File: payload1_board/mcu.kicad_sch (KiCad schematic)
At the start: 34 parts, among them U1 STM32WLE5CCU6, Y1 32.768KHz, Y2 32MHz

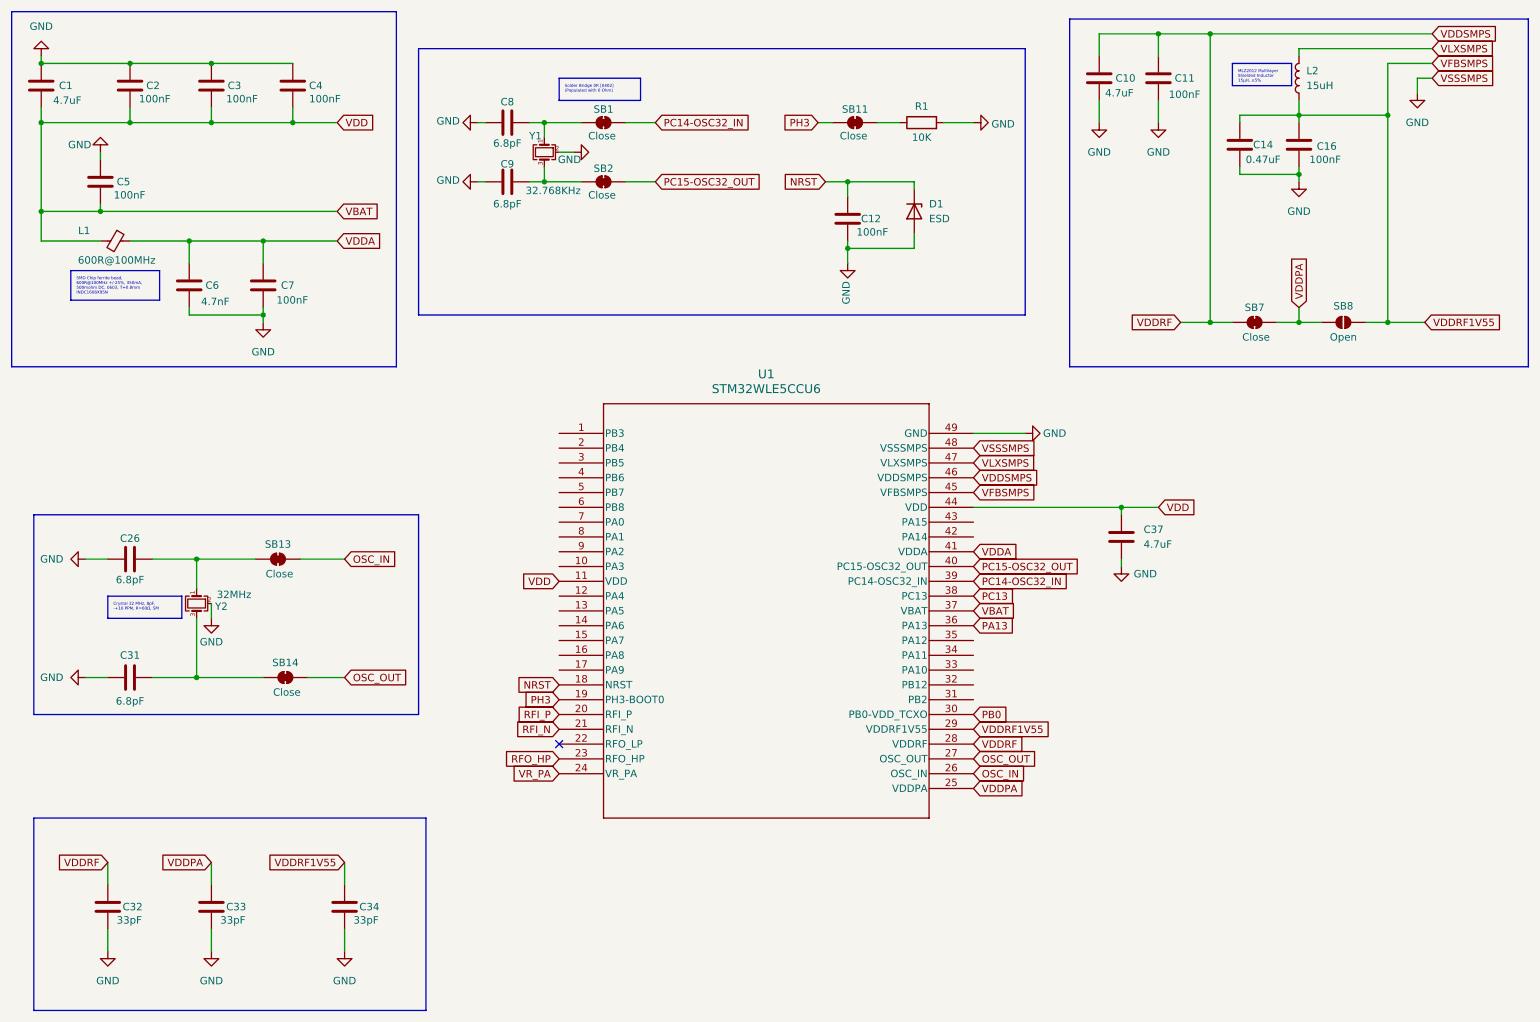
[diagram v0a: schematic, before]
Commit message: sensors done
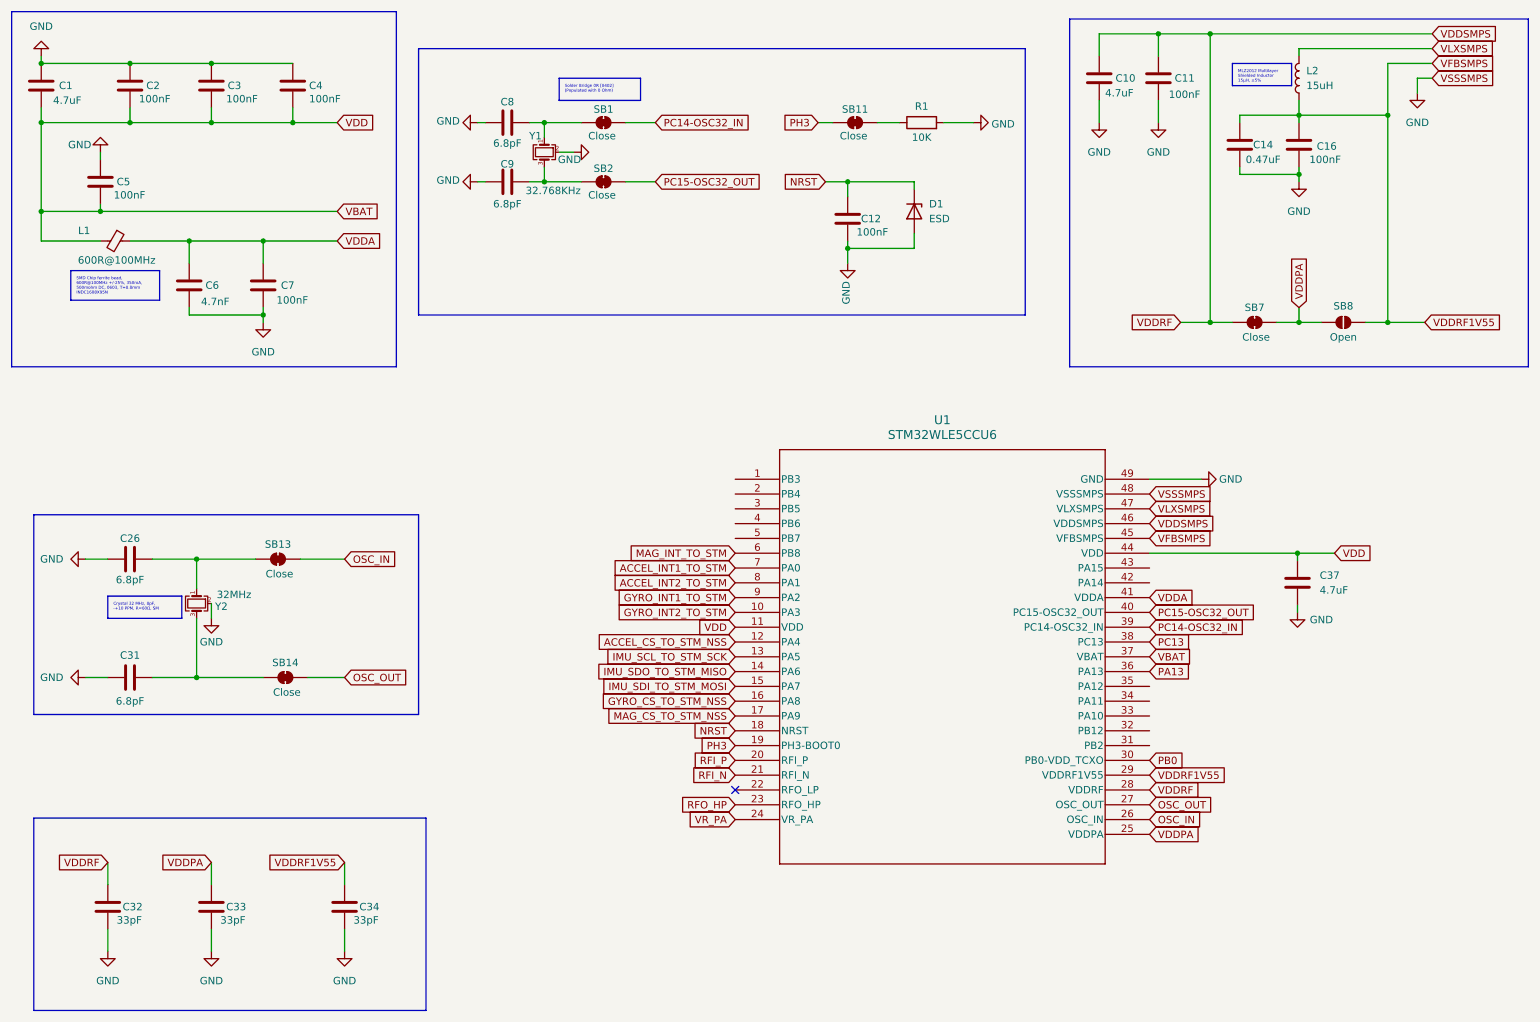
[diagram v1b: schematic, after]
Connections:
- net GYRO_INT2_TO_STM: now reaches U1.10 (PA3)
- net ACCEL_CS_TO_STM_NSS: now reaches U1.12 (PA4)
- net IMU_SCL_TO_STM_SCK: now reaches U1.13 (PA5)
- net IMU_SDO_TO_STM_MISO: now reaches U1.14 (PA6)
- net IMU_SDI_TO_STM_MOSI: now reaches U1.15 (PA7)
- net GYRO_CS_TO_STM_NSS: now reaches U1.16 (PA8)
- net MAG_CS_TO_STM_NSS: now reaches U1.17 (PA9)
- net MAG_INT_TO_STM: now reaches U1.6 (PB8)
- net ACCEL_INT1_TO_STM: now reaches U1.7 (PA0)
- net ACCEL_INT2_TO_STM: now reaches U1.8 (PA1)
- net GYRO_INT1_TO_STM: now reaches U1.9 (PA2)
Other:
- moved on the sheet: C37, U1
